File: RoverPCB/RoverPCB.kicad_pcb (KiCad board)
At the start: 2 copper layers, 78 x 82.3 mm, 24 parts, among them J1 Conn_01x02, J10 Conn_01x04_Pin, J11 Conn_01x04_Pin, J12 Conn_01x04_Pin, J13 Conn_01x04_Pin, J14 Conn_01x04_Pin, J15 Conn_01x04_Pin, J16 Conn_01x04_Pin, J17 Conn_01x04_Pin, J2 Conn_01x04_Pin, J3 Conn_01x04_Pin, J4 Conn_01x06_Pin, J5 Conn_01x15_Socket, J6 Conn_01x04_Pin, J7 Conn_01x04_Pin, J8 Conn_01x04_Pin, J9 Conn_01x04_Pin

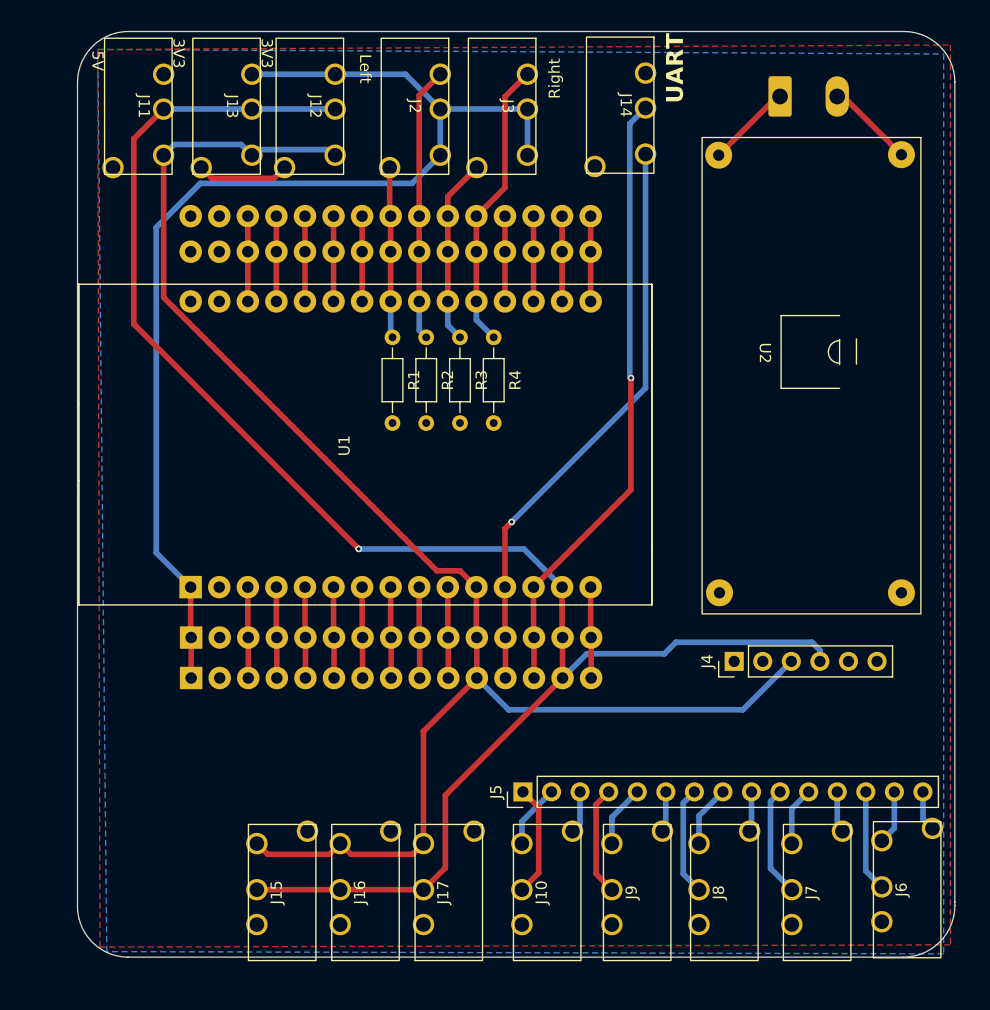
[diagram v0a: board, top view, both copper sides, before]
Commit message: PCBs
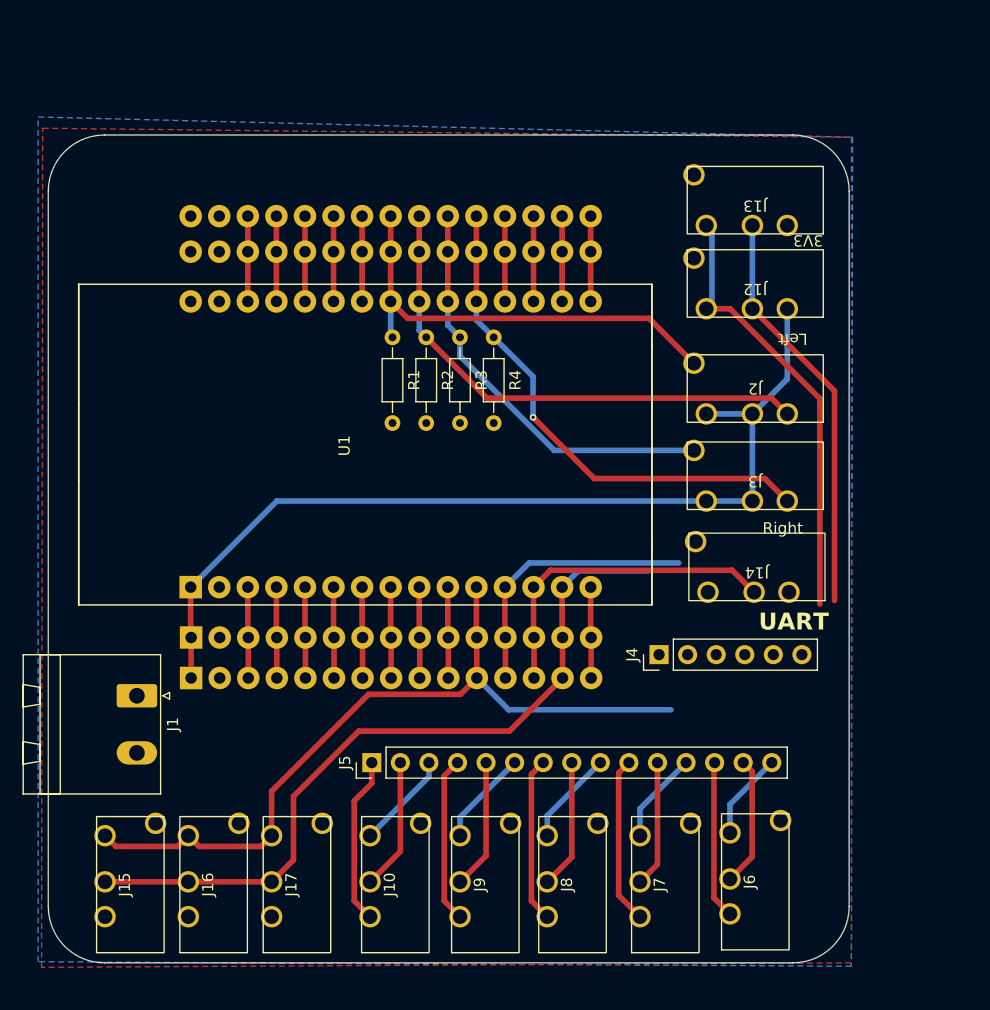
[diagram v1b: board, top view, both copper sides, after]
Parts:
- removed J11: Conn_01x04_Pin, Meloen:Audio jack
- removed U2: ~, Zuydlib3:LM2596_module
- J1: moved to F.Cu
- moved J1 78.2 mm to (36.3, 77.1), turned to -90 degrees
- moved J13 47.7 mm to (91.2, 33.0), turned to 180 degrees
- moved J14 42.8 mm to (91.4, 65.6), turned to 180 degrees
- moved J12 42.6 mm to (91.2, 40.4), turned to 180 degrees
- moved J3 39.8 mm to (91.2, 57.5), turned to 180 degrees
- moved J2 39.3 mm to (91.2, 49.7), turned to 180 degrees
- moved J5 13.7 mm to (57.2, 83.0)
- moved J15 13.5 mm to (35.7, 93.8)
- moved J16 13.5 mm to (43.1, 93.8)
- moved J6 13.5 mm to (91.3, 93.6)
- moved J7 13.5 mm to (83.3, 93.8)
- moved J8 13.5 mm to (75.0, 93.8)
- moved J9 13.5 mm to (67.3, 93.8)
- moved J10 13.5 mm to (59.3, 93.8)
- moved J17 13.5 mm to (50.5, 93.8)
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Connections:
- J1 pad 1: Net-(J1-Pin_1) -> GND
- J1 pad 2: Net-(J1-Pin_2) -> +5V
- J10 pad 1: GND -> Net-(J10-Pin_1)
- J10 pad 4: Net-(J10-Pin_4) -> GND
- J13 pad 1: +3V3 -> +5V
- J5 pad 1: Net-(J10-Pin_2) -> Net-(J10-Pin_1)
- J5 pad 2: Net-(J10-Pin_3) -> Net-(J10-Pin_2)
- J5 pad 3: Net-(J10-Pin_4) -> Net-(J10-Pin_3)
- J6 pad 1: GND -> Net-(J5-Pin_13)
- J6 pad 2: Net-(J5-Pin_13) -> Net-(J5-Pin_14)
- J6 pad 3: Net-(J5-Pin_14) -> Net-(J5-Pin_15)
- J6 pad 4: Net-(J5-Pin_15) -> GND
- J7 pad 1: GND -> Net-(J5-Pin_10)
- J7 pad 2: Net-(J5-Pin_10) -> Net-(J5-Pin_11)
- J7 pad 3: Net-(J5-Pin_11) -> Net-(J5-Pin_12)
- J7 pad 4: Net-(J5-Pin_12) -> GND
- J8 pad 1: GND -> Net-(J5-Pin_7)
- J8 pad 2: Net-(J5-Pin_7) -> Net-(J5-Pin_8)
- J8 pad 3: Net-(J5-Pin_8) -> Net-(J5-Pin_9)
- J8 pad 4: Net-(J5-Pin_9) -> GND
- J9 pad 1: GND -> Net-(J5-Pin_4)
- J9 pad 2: Net-(J5-Pin_4) -> Net-(J5-Pin_5)
- J9 pad 3: Net-(J5-Pin_5) -> Net-(J5-Pin_6)
- J9 pad 4: Net-(J5-Pin_6) -> GND
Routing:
- net SCL: track 155.6 -> 104.2 mm, vias 1 -> 0
- net SDA: track 139.7 -> 108.8 mm
- net RX: track 51.8 -> 24.4 mm, vias 1 -> 0
- net TX: track 54.9 -> 29.1 mm, vias 1 -> 0
- net LDR1: track 15.9 -> 40.9 mm
- net Button1: track 24.4 -> 45.9 mm
- net LDR2: track 16.6 -> 37.2 mm
- net Button2: track 25.9 -> 45.7 mm, vias 0 -> 1
- net +3V3: track 103.2 -> 83.7 mm
- net Net-(J10-Pin_1): track 0.00 -> 14.9 mm
- net Net-(J1-Pin_2): track 7.86 -> 0.00 mm
- net Net-(J1-Pin_1): track 7.62 -> 0.00 mm
- net GND: track 8.19 -> 1.31 mm
- net Net-(J5-Pin_14): track 4.81 -> 11.5 mm
- net Net-(J5-Pin_11): track 5.22 -> 11.2 mm
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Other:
- board size 78 x 82.3 mm -> 71.2 x 73.6 mm
- board text removed: "5V"

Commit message: PCBRover final
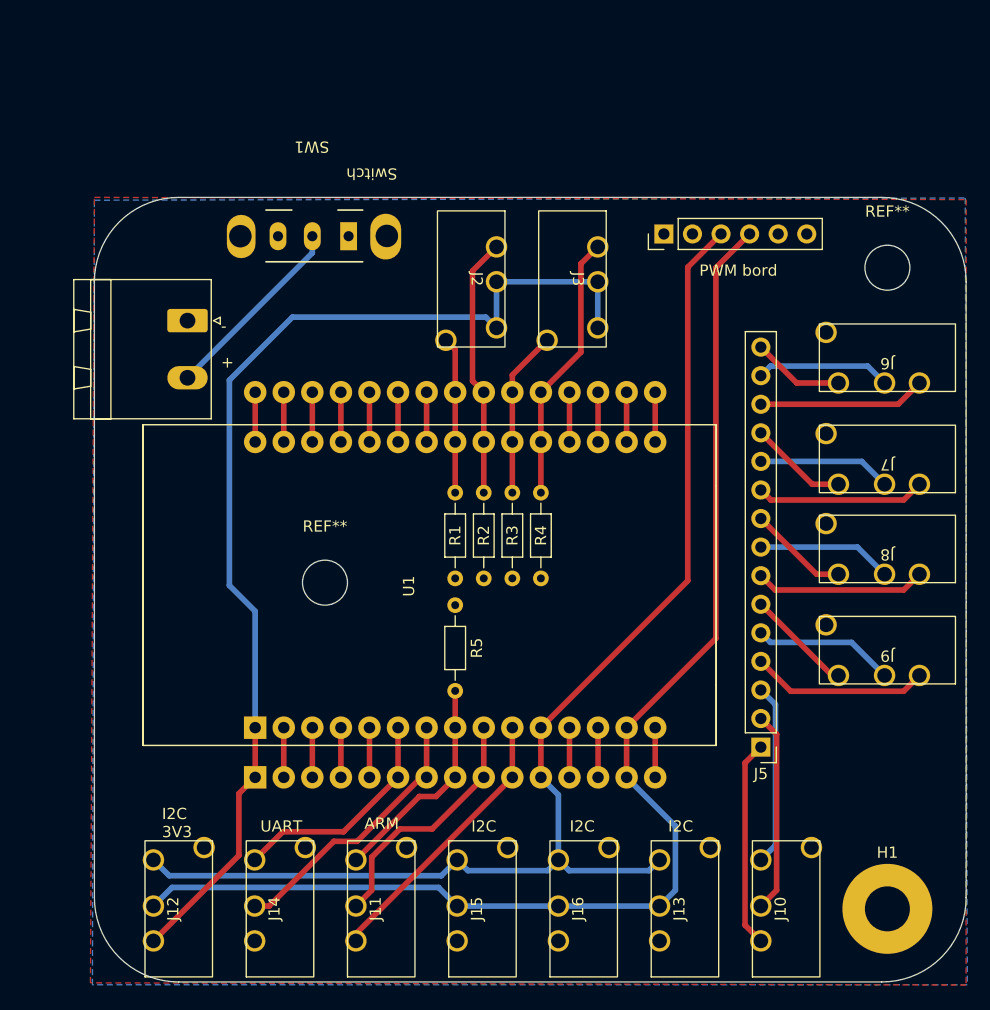
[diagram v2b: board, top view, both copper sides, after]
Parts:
- removed J17: Conn_01x04_Pin, Meloen:Audio jack
- added H1: MountingHole_Pad, MountingHole:MountingHole_4mm_Pad, F.Cu at (103.0, 96.0)
- added J11: arm, Meloen:Audio jack, F.Cu at (58.0, 96.0)
- added R5: R, Resistor_THT:R_Axial_DIN0204_L3.6mm_D1.6mm_P7.62mm_Horizontal, F.Cu at (64.6, 69.0)
- added REF**: MountingHole_4mm, MountingHole:MountingHole_4mm, F.Cu at (53.0, 67.0)
- added REF**: MountingHole_4mm, MountingHole:MountingHole_4mm, F.Cu at (103.0, 39.0)
- added SW1: SW_DPDT_x2, Zuydlib4:SW_CuK_SPDT_Angled, F.Cu at (51.8, 27.8)
- J1: value Conn_01x02 -> Voeding
- J10: value Conn_01x04_Pin -> ExtraPWM2
- J12: value Conn_01x04_Pin -> I2C 3V3
- J13, J15, J16: value Conn_01x04_Pin -> I2C
- J14: value Conn_01x04_Pin -> UART
- J2: value Conn_01x04_Pin -> Left solartacker
- J3: value Conn_01x04_Pin -> Right solartracker
- J4: value Conn_01x06_Pin -> PWM bord
- J6: value Conn_01x04_Pin -> Motor1
- J7: value Conn_01x04_Pin -> Motor2
- J8: value Conn_01x04_Pin -> Motor3
- J9: value Conn_01x04_Pin -> extraPWM1
- U1: footprint Meloen:ESP32_DEVKIT_V1_op_voetjes -> Meloen:ESP32_DEVKIT_V1_op_voetjes2rij
- moved J12 75.6 mm to (40.0, 96.0), turned to 90 degrees
- moved J13 63.3 mm to (85.0, 96.0), turned to 90 degrees
- moved J14 52.2 mm to (49.0, 96.0), turned to 90 degrees
- moved J6 48.1 mm to (103.0, 47.0), turned to 180 degrees
- moved J7 42.7 mm to (103.0, 56.0), turned to 180 degrees
- moved J9 41.4 mm to (103.0, 73.0), turned to 180 degrees
- moved J8 40.9 mm to (103.0, 64.0), turned to 180 degrees
- moved J4 37.4 mm to (83.1, 36.0)
- moved J10 34.8 mm to (94.0, 96.0)
- moved J5 34.6 mm to (91.8, 81.6), turned to 180 degrees
- moved J1 33.7 mm to (40.8, 43.7)
- moved J16 33.0 mm to (76.0, 96.0)
- moved J15 31.4 mm to (67.0, 96.0)
- moved J2 27.1 mm to (66.0, 40.0), turned to -90 degrees
- moved J3 23.9 mm to (75.0, 40.0), turned to -90 degrees
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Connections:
- J1 pad 2: +5V -> Net-(J1-Pin_2)
- U1 pad 10: unconnected-(U1-D19-Pad10) -> Transistor metaal
- U1 pad 12: RX -> unconnected-(U1-RX0-Pad12)
- U1 pad 13: TX -> unconnected-(U1-TX0-Pad13)
- U1 pad 6: unconnected-(U1-RX2-Pad6) -> RX
- U1 pad 7: unconnected-(U1-TX2-Pad7) -> TX
- U1 pad 8: unconnected-(U1-D5-Pad8) -> Metaal detector
- U1 pad 9: unconnected-(U1-D18-Pad9) -> Transistor magneet
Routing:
- net LDR1: track 40.9 -> 13.9 mm
- net Transistor metaal: track 0.00 -> 24.7 mm
- net Button1: track 45.9 -> 23.1 mm
- net LDR2: track 37.2 -> 14.8 mm
- net Transistor magneet: track 0.00 -> 22.2 mm
- net Button2: track 45.7 -> 23.9 mm, vias 1 -> 0
- net Metaal detector: track 0.00 -> 19.6 mm
- net Net-(J1-Pin_2): track 0.00 -> 17.2 mm
- net +3V3: track 83.7 -> 98.2 mm
- net SCL: track 104.2 -> 113.0 mm
- net unconnected-(U1-TX2-Pad7): track 8.09 -> 0.00 mm
- net unconnected-(U1-RX2-Pad6): track 8.09 -> 0.00 mm
- net unconnected-(U1-D5-Pad8): track 8.09 -> 0.00 mm
- net unconnected-(U1-D19-Pad10): track 8.09 -> 0.00 mm
- net unconnected-(U1-D18-Pad9): track 8.09 -> 0.00 mm
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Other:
- board size 71.2 x 73.6 mm -> 77.5 x 69.8 mm
- board text added: "- +"
- board text added: "ARM"
- board text added: "I2C"
- board text added: "I2C 3V3"
- board text removed: "3V3"
- board text removed: "Koen Aben Solar Rover"
- board text removed: "Left"
- board text removed: "Right"

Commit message: PowerPCB
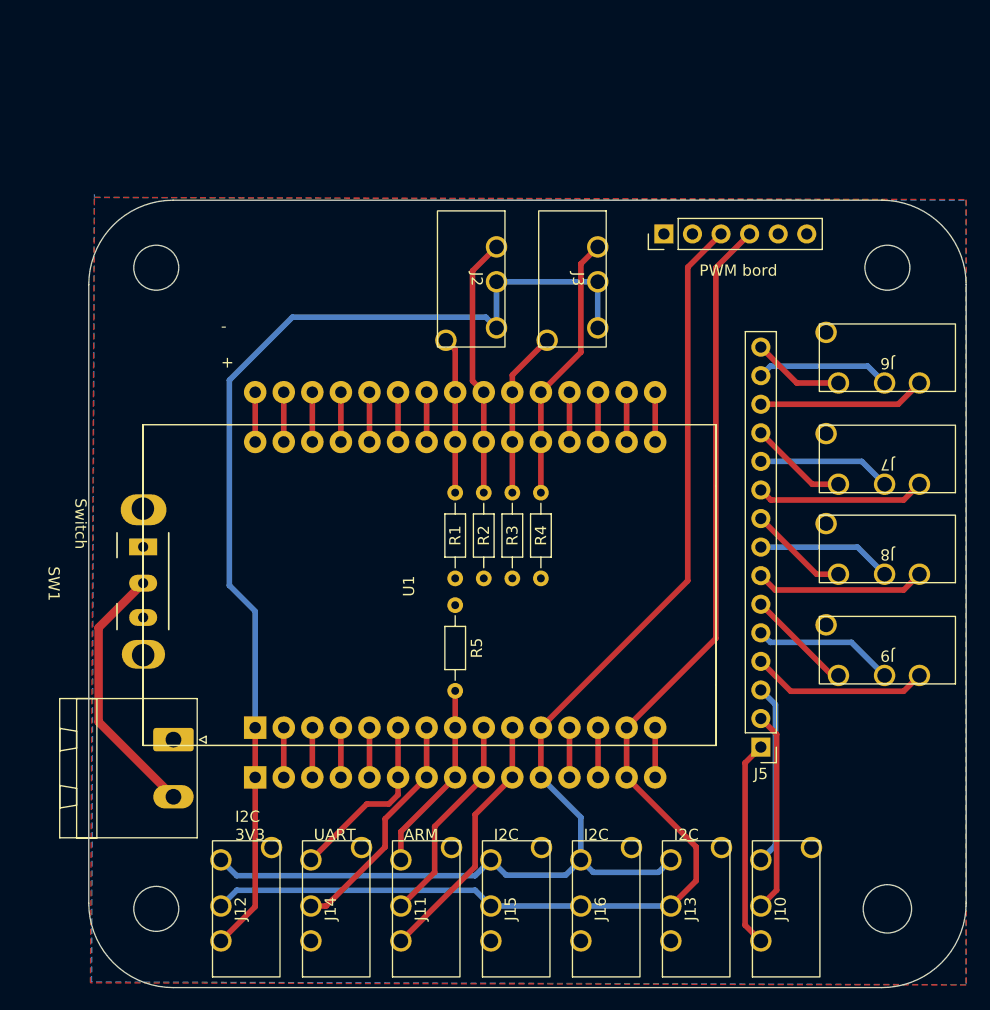
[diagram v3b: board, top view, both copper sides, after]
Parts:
- removed H1: MountingHole_Pad, MountingHole:MountingHole_4mm_Pad
- added REF**: MountingHole_4mm, MountingHole:MountingHole_4mm, F.Cu at (38.0, 39.0)
- added REF**: MountingHole_4.3mm_M4, MountingHole:MountingHole_4.3mm_M4, F.Cu at (103.0, 96.0)
- moved SW1 45.8 mm to (28.4, 67.1), turned to -90 degrees
- moved J1 37.3 mm to (39.5, 81.0)
- moved REF** 32.6 mm to (38.0, 96.0)
- moved J12 6.00 mm to (46.0, 96.0)
- moved J14 5.00 mm to (54.0, 96.0)
- moved J11 4.00 mm to (62.0, 96.0)
- moved J15 3.00 mm to (70.0, 96.0)
- moved J16 2.00 mm to (78.0, 96.0)
- moved J13 1.00 mm to (86.0, 96.0)
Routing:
- net Net-(J1-Pin_2): track 17.2 -> 23.4 mm
- net RX: track 20.2 -> 16.1 mm
- net SCL: track 113.0 -> 108.9 mm
- net SDA: track 110.7 -> 106.9 mm
- net Transistor magneet: track 22.2 -> 18.9 mm
- net TX: track 24.4 -> 21.4 mm
- net Metaal detector: track 19.6 -> 17.0 mm
- net +3V3: track 98.2 -> 95.7 mm
- net Transistor metaal: track 24.7 -> 23.1 mm
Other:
- board size 77.5 x 69.8 mm -> 78 x 70 mm
